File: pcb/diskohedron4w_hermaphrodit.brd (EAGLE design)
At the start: 94.1 x 58.1 mm, 23 parts

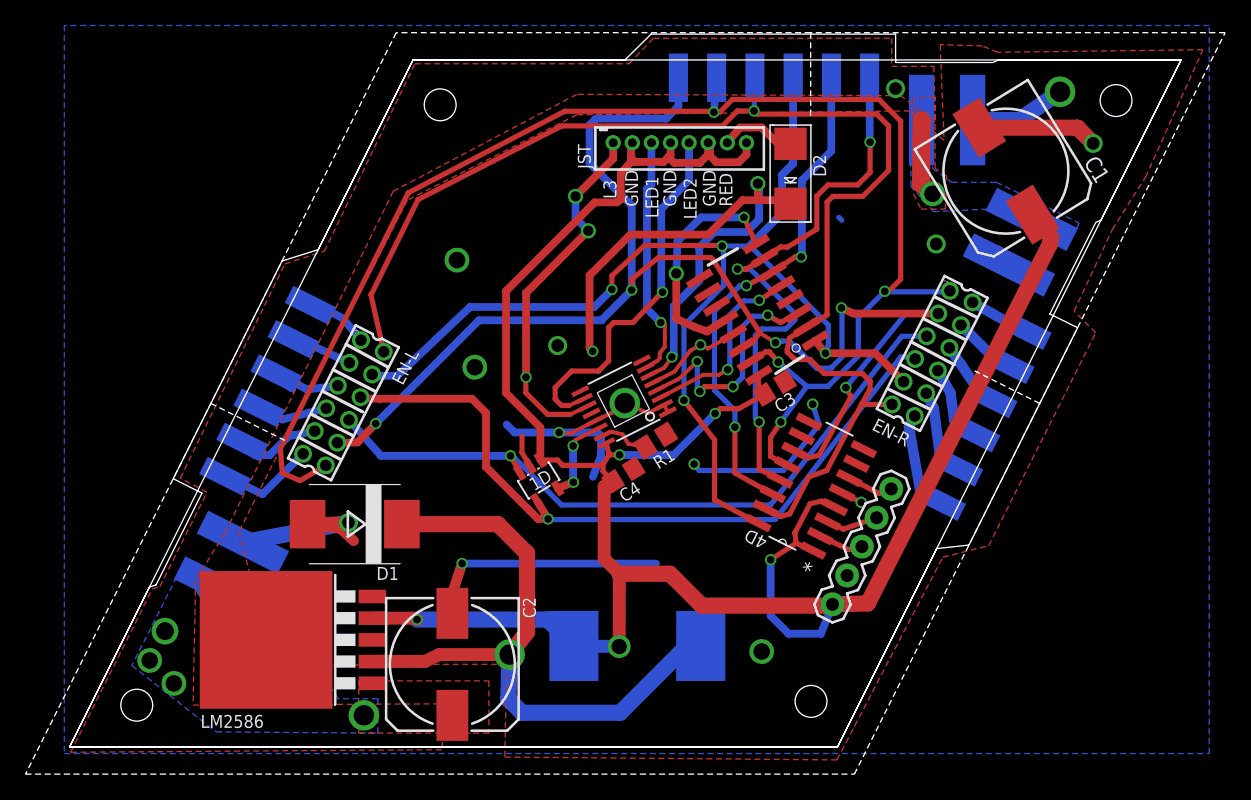
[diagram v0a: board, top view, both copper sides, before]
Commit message: order for itead 12/05/2014 #100029337
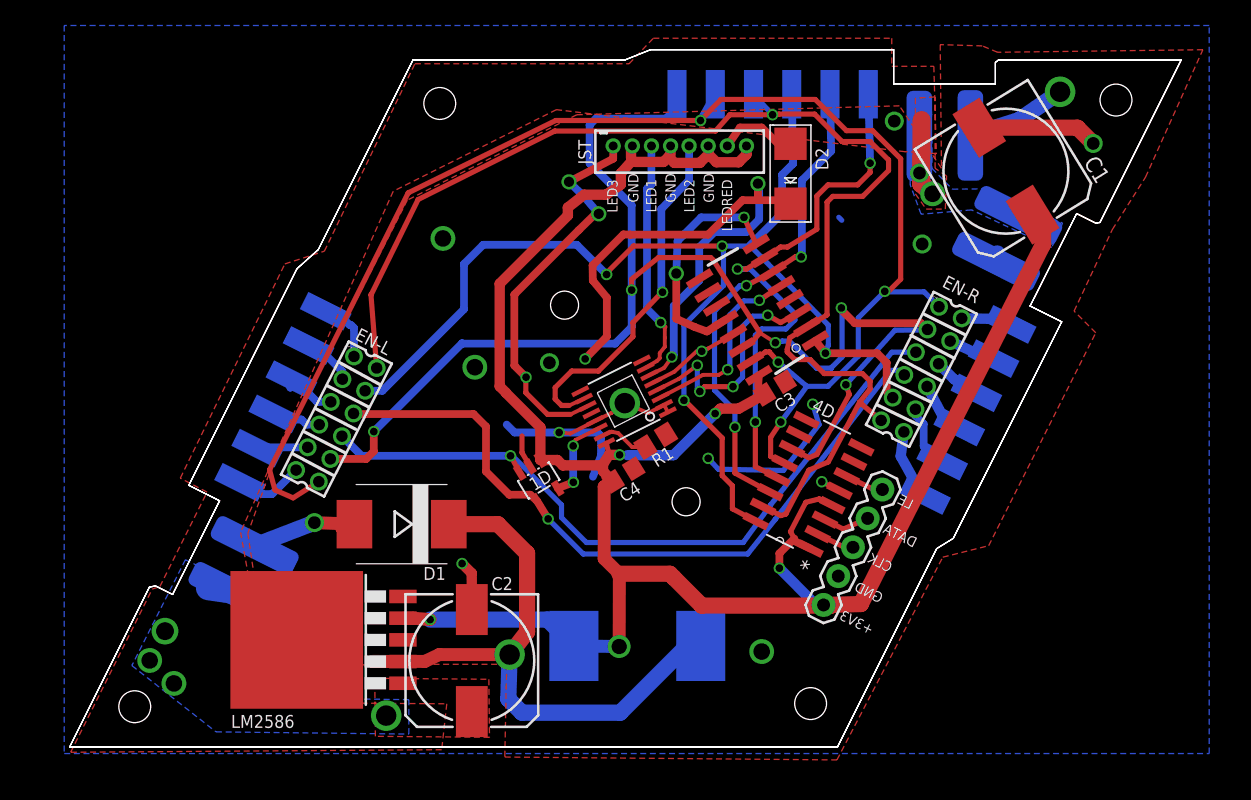
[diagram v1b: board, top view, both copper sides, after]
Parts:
- R1: value 220r -> 220R
- moved D1 3.68 mm to (26.1, 17.5)
- moved LM2586 2.40 mm to (20.4, 8.41)
- moved U$7 1.76 mm to (72.6, 44.5)
- moved U$6 1.59 mm to (68.7, 38.0)
- moved C2 1.55 mm to (31.6, 6.79)
- moved EN-R 1.51 mm to (66.8, 29.6)
- moved U$12 1.50 mm to (18.5, 15.9)
- moved EN-L 1.39 mm to (20.9, 25.7)
- moved IN1 1.30 mm to (64.7, 49.8)
- moved OUT-R 1.28 mm to (65.0, 18.6)
- moved OUT-L 1.27 mm to (22.3, 35.3)
- moved JP1 0.70 mm to (59.2, 11.2)
- moved 4D 0.25 mm to (57.8, 25.7)
- moved JST 0.25 mm to (44.9, 47.2)
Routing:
- net GND: track 113.5 -> 94.0 mm
- net +3V3: track 180.3 -> 172.0 mm
- net CLK-: track 94.3 -> 98.2 mm
- net OE+L: track 6.79 -> 3.97 mm
- net +24V: track 8.04 -> 10.5 mm, vias 6 -> 7
- net LED3: track 29.0 -> 31.4 mm
- net OE-L: track 7.74 -> 5.40 mm
- net CLK+R: track 7.87 -> 5.95 mm
- net N$3: track 45.9 -> 47.7 mm
- net DATAOUT+R: track 6.05 -> 4.23 mm
- net DATAOUT-L: track 5.58 -> 3.83 mm
- net DATAOUT-: track 56.2 -> 57.8 mm
- net DATA+: track 40.3 -> 38.8 mm
- net DATA-: track 44.6 -> 43.1 mm
- net N$2: track 51.3 -> 50.0 mm
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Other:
- board size 94.1 x 58.1 mm -> 87.2 x 54.7 mm
- board text added: "05/2014"
- board text added: "DISKO HEDRON"
- board text added: "LED3"
- board text added: "LEDRED"
- board text added: "SAVIC LAMMER SAVICIC"
- board text added: "rev.A"
- board text removed: "L3"
- board text removed: "RED"
